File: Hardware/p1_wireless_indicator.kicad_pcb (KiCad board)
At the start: 4 copper layers, 50.7 x 40 mm, 42 parts, among them J1 615006138421, J2 629722000214, SW1 KSEM31JLFS, SW2 KSEM31JLFS, U1 140357145100, U2 140357145100, U3 173950336, U4 ESP32-C3-WROOM-02-N4

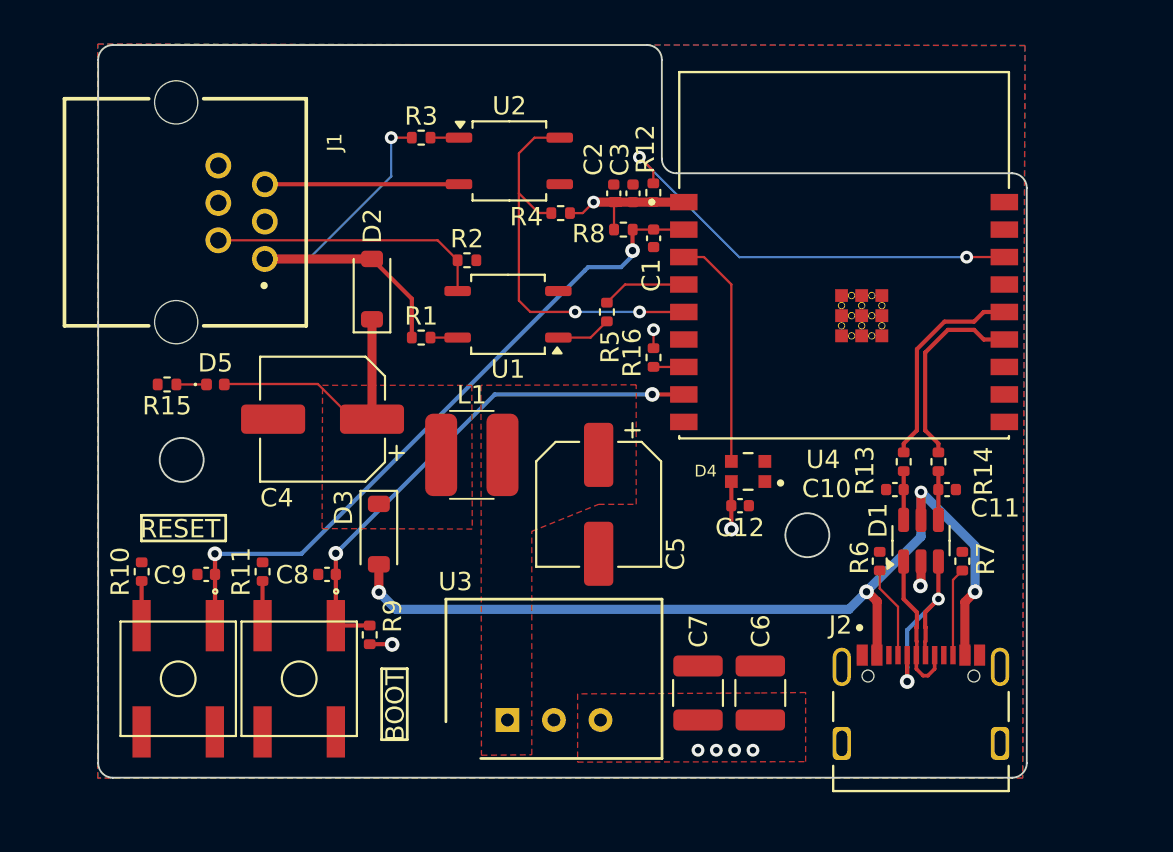
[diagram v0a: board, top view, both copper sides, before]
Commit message: Rounting of V2.0
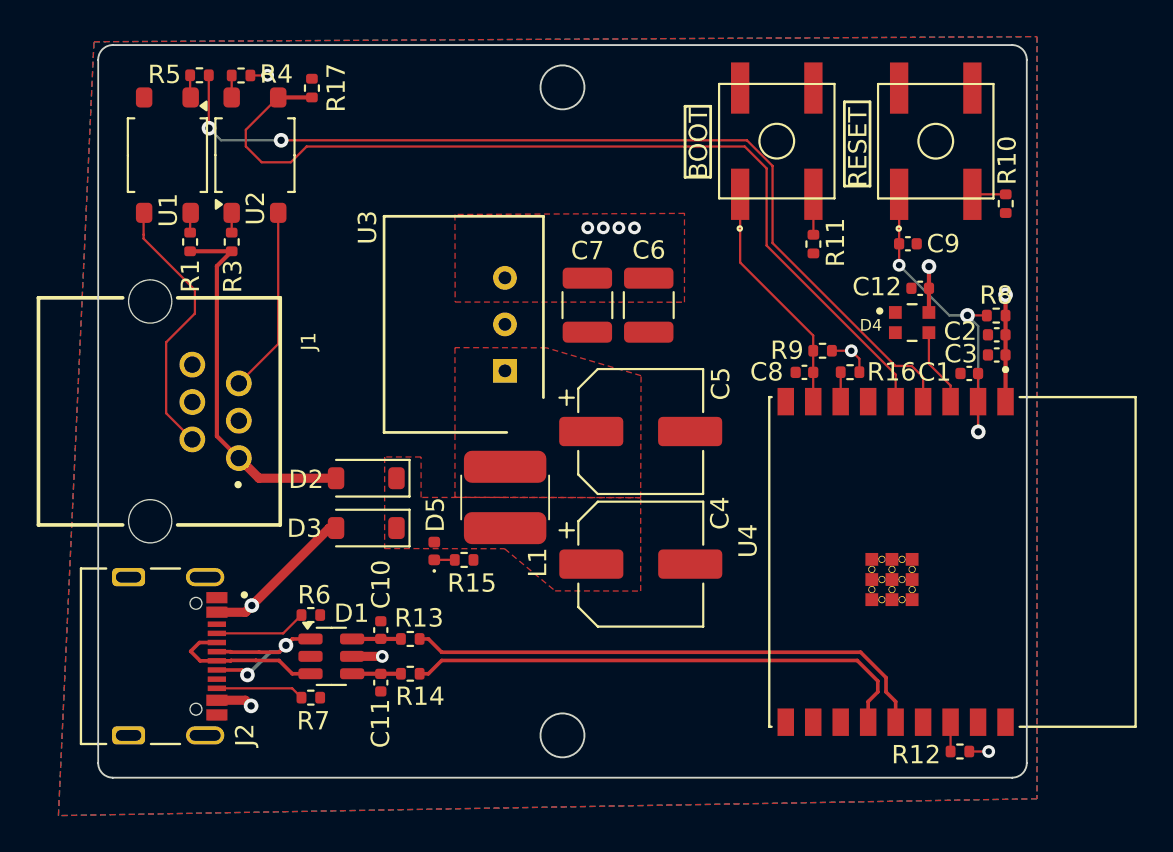
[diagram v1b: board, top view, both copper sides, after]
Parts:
- removed R2: 1M, Resistor_SMD:R_0402_1005Metric
- added R17: 1M, Resistor_SMD:R_0402_1005Metric, F.Cu at (104.6, 64.3)
- R3: value 1K -> 220R
- U1, U2: footprint Package_SO:SOP-4_3.8x4.1mm_P2.54mm -> manul_tech:140357145100
- moved R10 51.3 mm to (142.5, 70.7), turned to -90 degrees
- moved SW1 50.7 mm to (138.7, 67.2), turned to 90 degrees
- moved J2 43.5 mm to (94.6, 95.4), turned to -90 degrees
- moved C9 42.3 mm to (137.2, 72.8), turned to 180 degrees
- moved SW2 39.3 mm to (130.0, 67.2), turned to 90 degrees
- moved R7 36.3 mm to (104.6, 97.6), turned to 0 degrees
- moved R11 35.0 mm to (132.0, 72.9), turned to -90 degrees
- moved R12 34.8 mm to (140.0, 100.6), turned to 180 degrees
- moved D1 32.8 mm to (105.7, 95.4), turned to 0 degrees
- moved C11 32.7 mm to (108.4, 96.8), turned to -90 degrees
- moved R6 31.2 mm to (104.6, 93.1), turned to 180 degrees
- moved R14 31.1 mm to (110.0, 96.3), turned to 0 degrees
- moved R9 29.2 mm to (132.5, 78.7), turned to 180 degrees
- moved C10 29.1 mm to (108.4, 93.9), turned to 90 degrees
- moved R13 28.6 mm to (110.0, 94.4), turned to 0 degrees
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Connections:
- R4 pad 2: /RX -> Net-(R4-Pad2)
- U2 pad 3: GND -> /RX
- U2 pad 4: /RX -> Net-(R4-Pad2)
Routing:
- net /RTS: track 4.61 -> 51.8 mm, vias 0 -> 2
- net /RX: track 22.1 -> 50.5 mm, vias 2 -> 0
- net VBUS: track 51.3 -> 25.1 mm, vias 4 -> 3
- net Net-(U4-IO2): track 23.9 -> 1.60 mm, vias 2 -> 0
- net /EN: track 37.7 -> 19.6 mm, vias 2 -> 3
- net /DA+: track 11.5 -> 29.0 mm
- net /DA-: track 10.8 -> 28.2 mm
- net /BOOT: track 28.4 -> 13.0 mm, vias 2 -> 0
- net Net-(D2-K): track 14.3 -> 0.00 mm
- net /STATUS_LED: track 12.9 -> 4.26 mm
- net /D-: track 12.1 -> 8.70 mm, vias 2 -> 0
- net +5V: track 23.1 -> 20.2 mm, vias 1 -> 0
- net /D+: track 8.25 -> 9.98 mm, vias 0 -> 2
- net Net-(R4-Pad2): track 0.00 -> 1.60 mm
- net Net-(R5-Pad2): track 3.02 -> 1.62 mm
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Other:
- outline, holes or cut-outs redrawn
